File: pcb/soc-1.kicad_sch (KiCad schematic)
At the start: 1 part, among them U1 XC7Z020CLG484

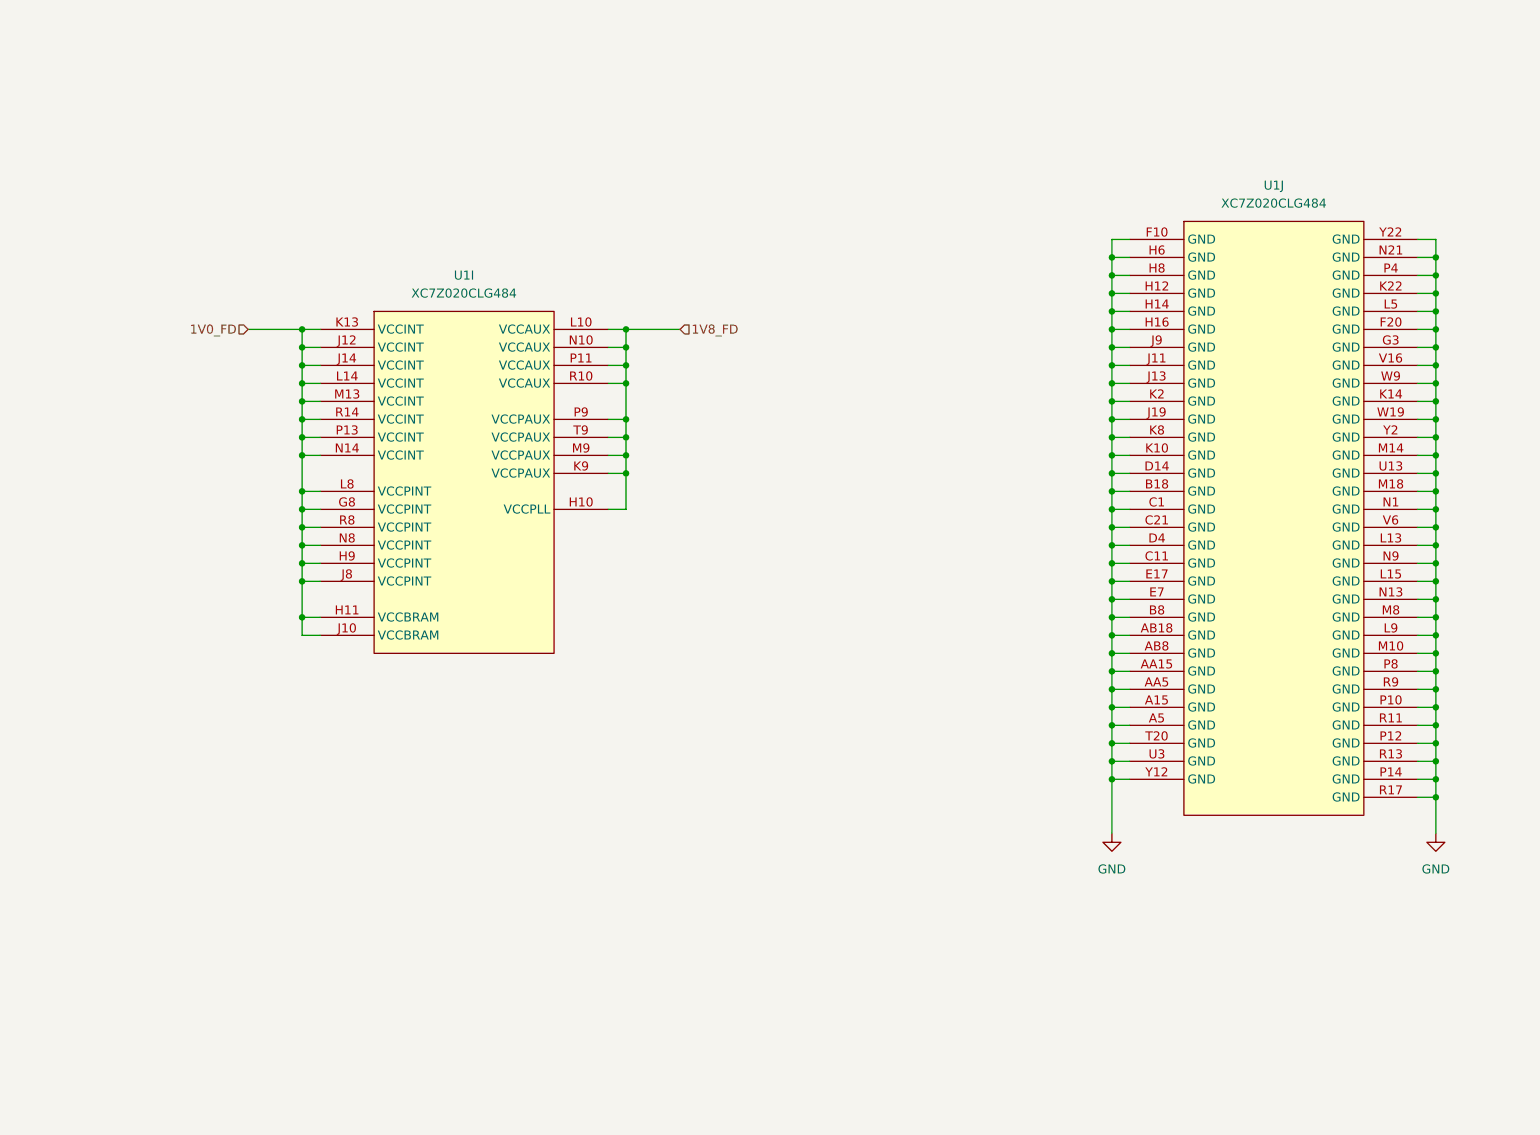
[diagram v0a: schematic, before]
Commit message: hierarchy and cleaning
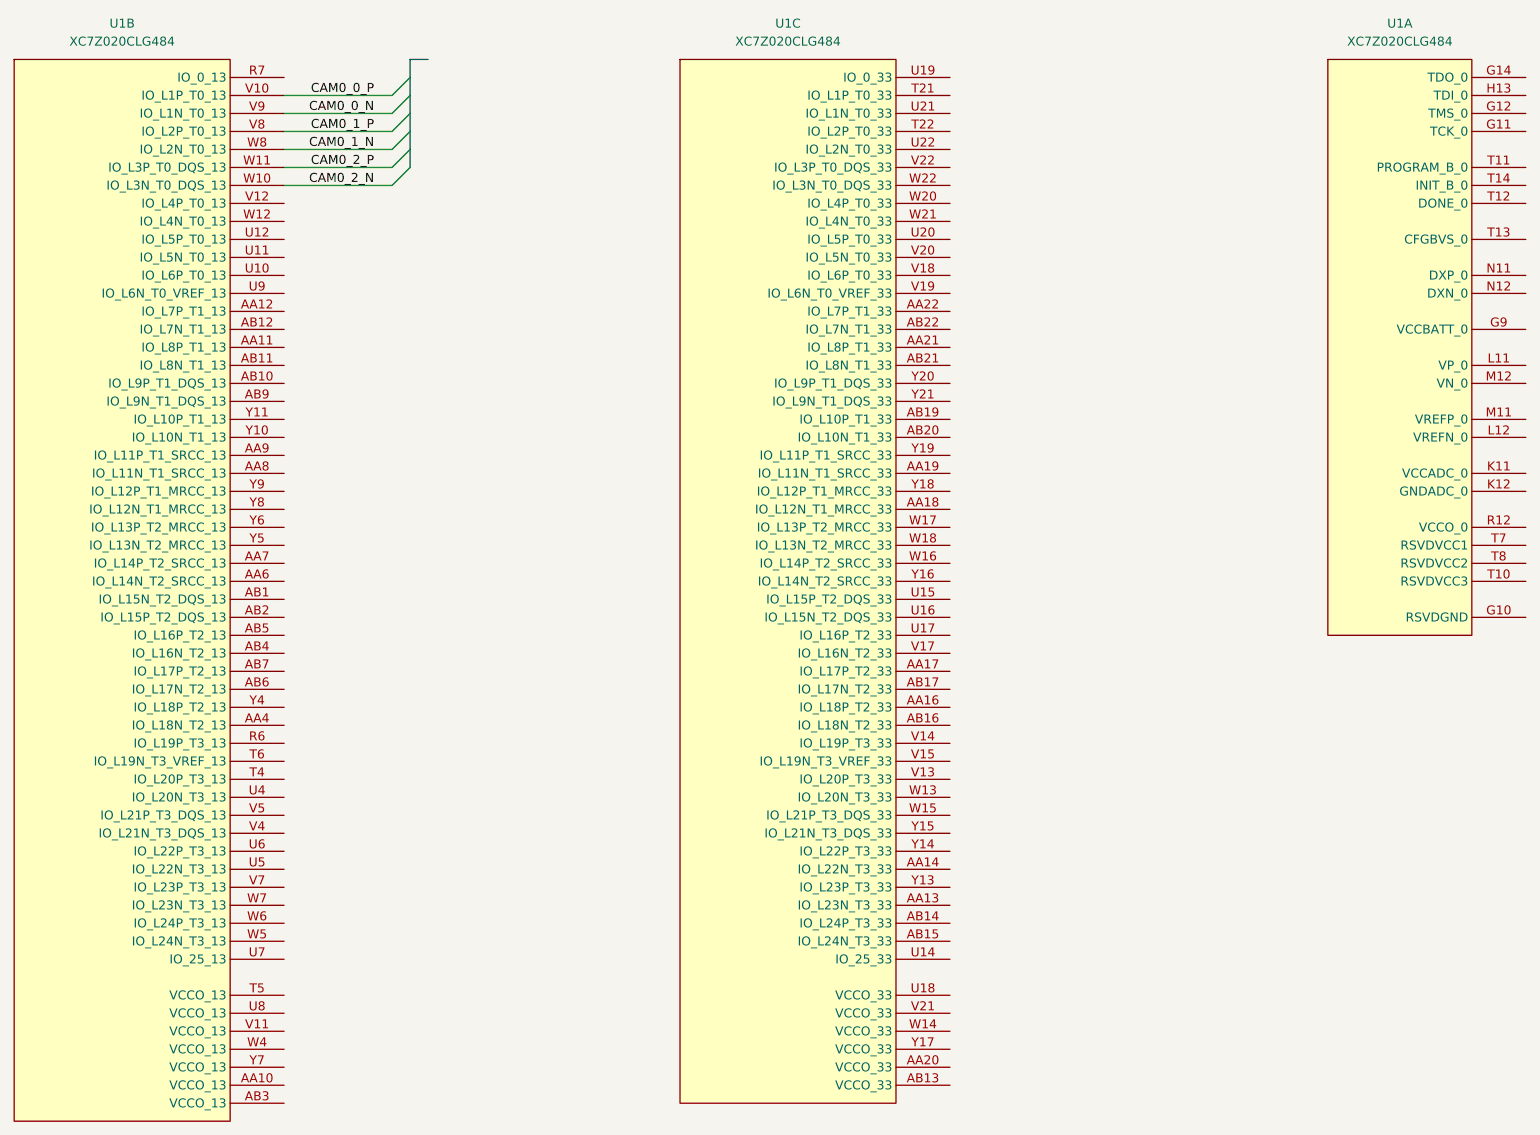
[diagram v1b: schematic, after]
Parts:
- removed U1: XC7Z020CLG484, Package_BGA:Xilinx_CLG484_CLG485, symbol library:XC7Z020CLG484
- added U1: XC7Z020CLG484, Package_BGA:Xilinx_CLG484_CLG485, symbol library:XC7Z020CLG484
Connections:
- new net CAM0_0_N: U1.V9 (IO_L1N_T0_13)
- new net CAM0_0_P: U1.V10 (IO_L1P_T0_13)
- new net CAM0_1_N: U1.W8 (IO_L2N_T0_13)
- new net CAM0_1_P: U1.V8 (IO_L2P_T0_13)
- new net CAM0_2_N: U1.W10 (IO_L3N_T0_DQS_13)
- new net CAM0_2_P: U1.W11 (IO_L3P_T0_DQS_13)
